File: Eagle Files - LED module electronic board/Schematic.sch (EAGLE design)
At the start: 14 parts, among them IC1 AMS1117-1.5, IC2 LM358N, J1 2.54 CONN, J2 2.54 CONN, Q1 P16NF06L

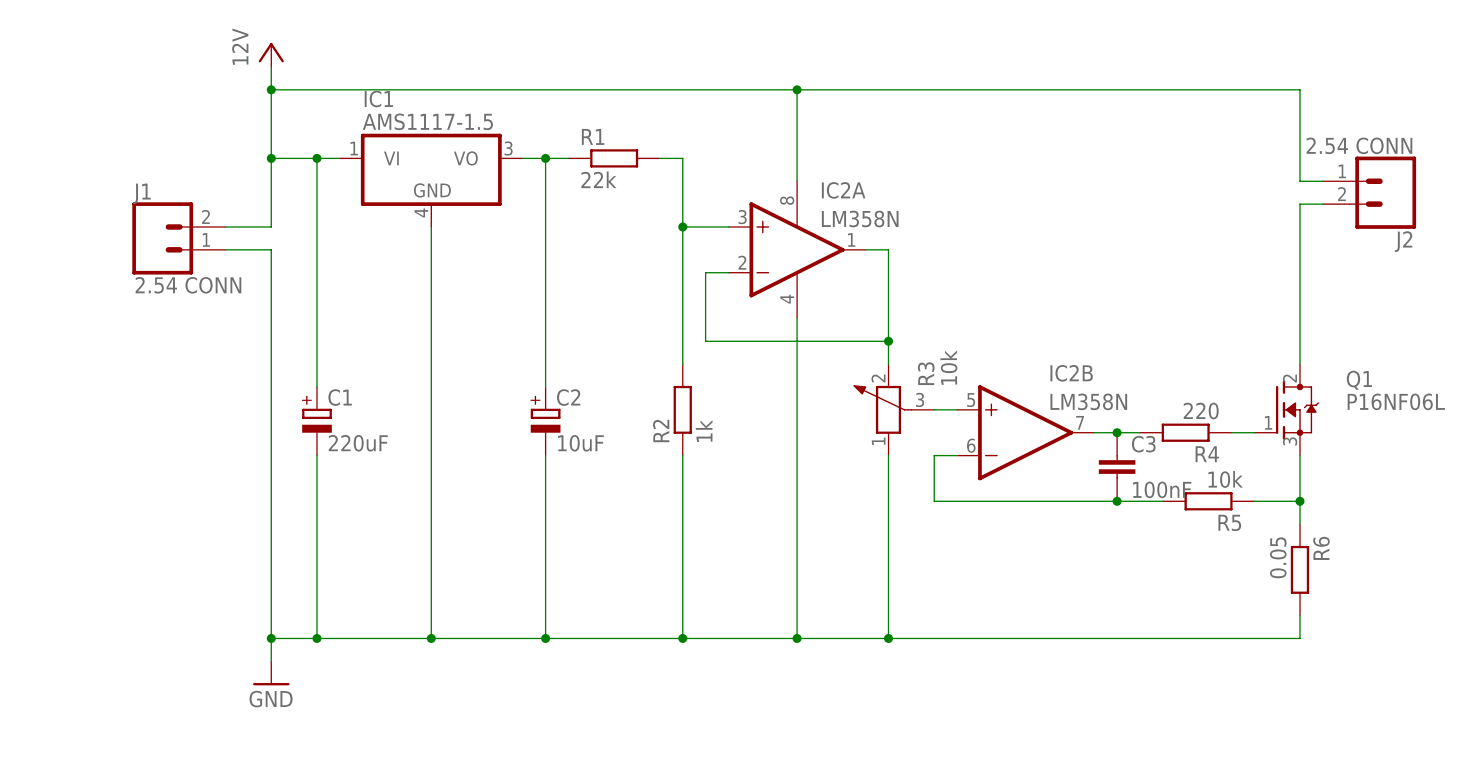
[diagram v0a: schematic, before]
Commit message: Update
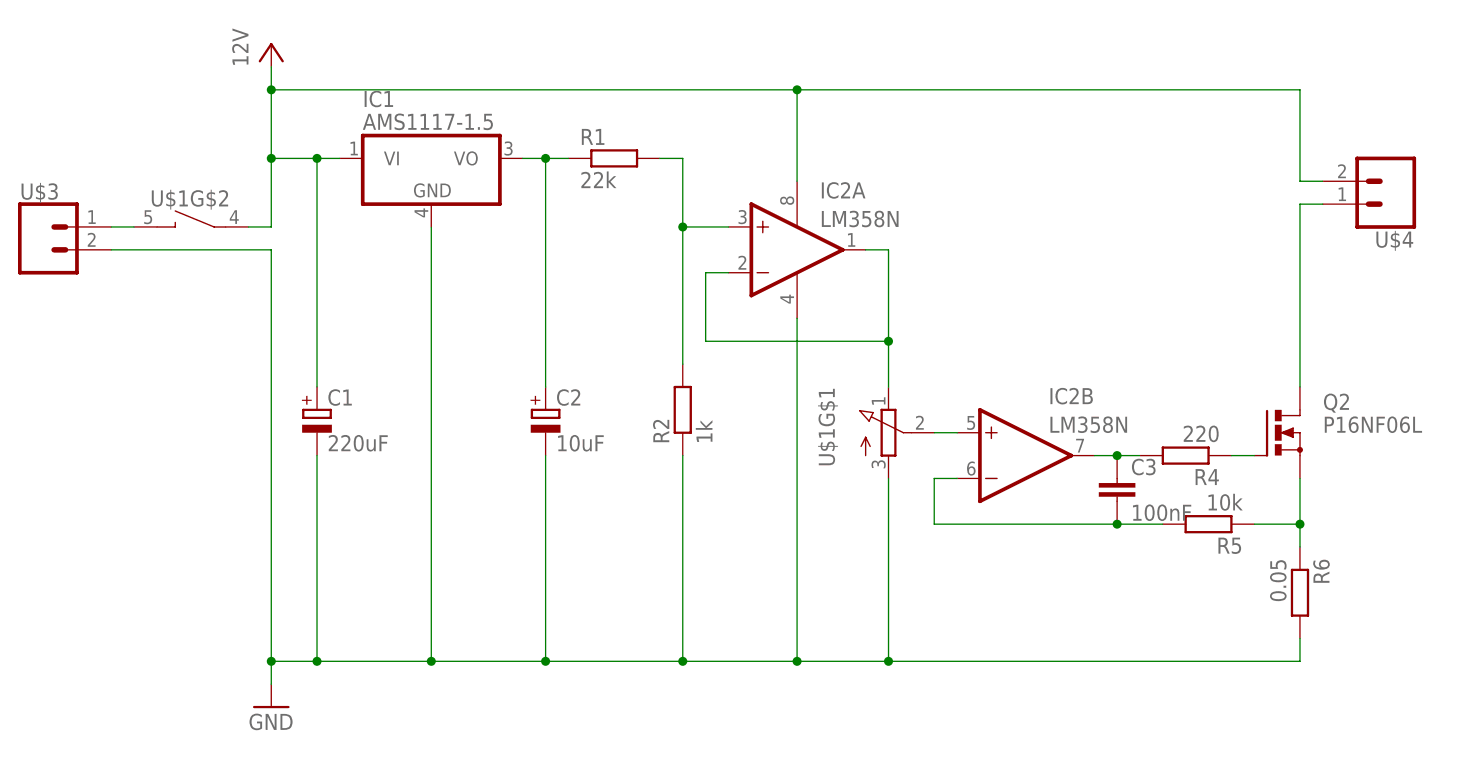
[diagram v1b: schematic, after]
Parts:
- removed J1, J2: 2.54 CONN, SparkFun-Connectors:CONN_02
- removed Q1: P16NF06L, adafruit:MOSFET-NGDS_TO220V
- removed R3: 10k, LED-microscope-library:POTENTIOMETER_3-PIN
- added Q2: P16NF06L, transistor-power:PMOSFET_NTO220BV
- added U$1: (no value), untitled:POT-SWITCH
- added U$3, U$4: (no value), untitled:SCREW-TERM
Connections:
- new net N$10: IC2B.+IN, U$1G$1.P$2
- net GND: now also U$1G$1.P$3, U$3.1; no longer J1.1, R3.1
- net N$1: now also U$1G$2.P$2, U$3.2; no longer IC2B.+IN, R3.3
- net N$4: now also U$1G$1.P$1; no longer R3.2
- net N$5: now also Q2.D, U$4.2; no longer J2.2, Q1.D
- net N$7: now also Q2.G; no longer Q1.G
- net N$9: now also Q2.S; no longer Q1.S
- net VCC: now also U$1G$2.P$1, U$4.1; no longer J1.2, J2.1
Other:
- moved on the sheet: C3, IC2B, R4, R5, R6
